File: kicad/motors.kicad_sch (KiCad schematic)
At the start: 61 parts, among them J12 Conn_01x04_Pin, J3 Conn_01x04_Pin, J4 Conn_01x04_Pin, J5 Conn_01x04_Pin, J6 Conn_01x04_Pin, U3 DRV8825PWP, U4 DRV8825PWP, U5 DRV8825PWP, U6 DRV8825PWP

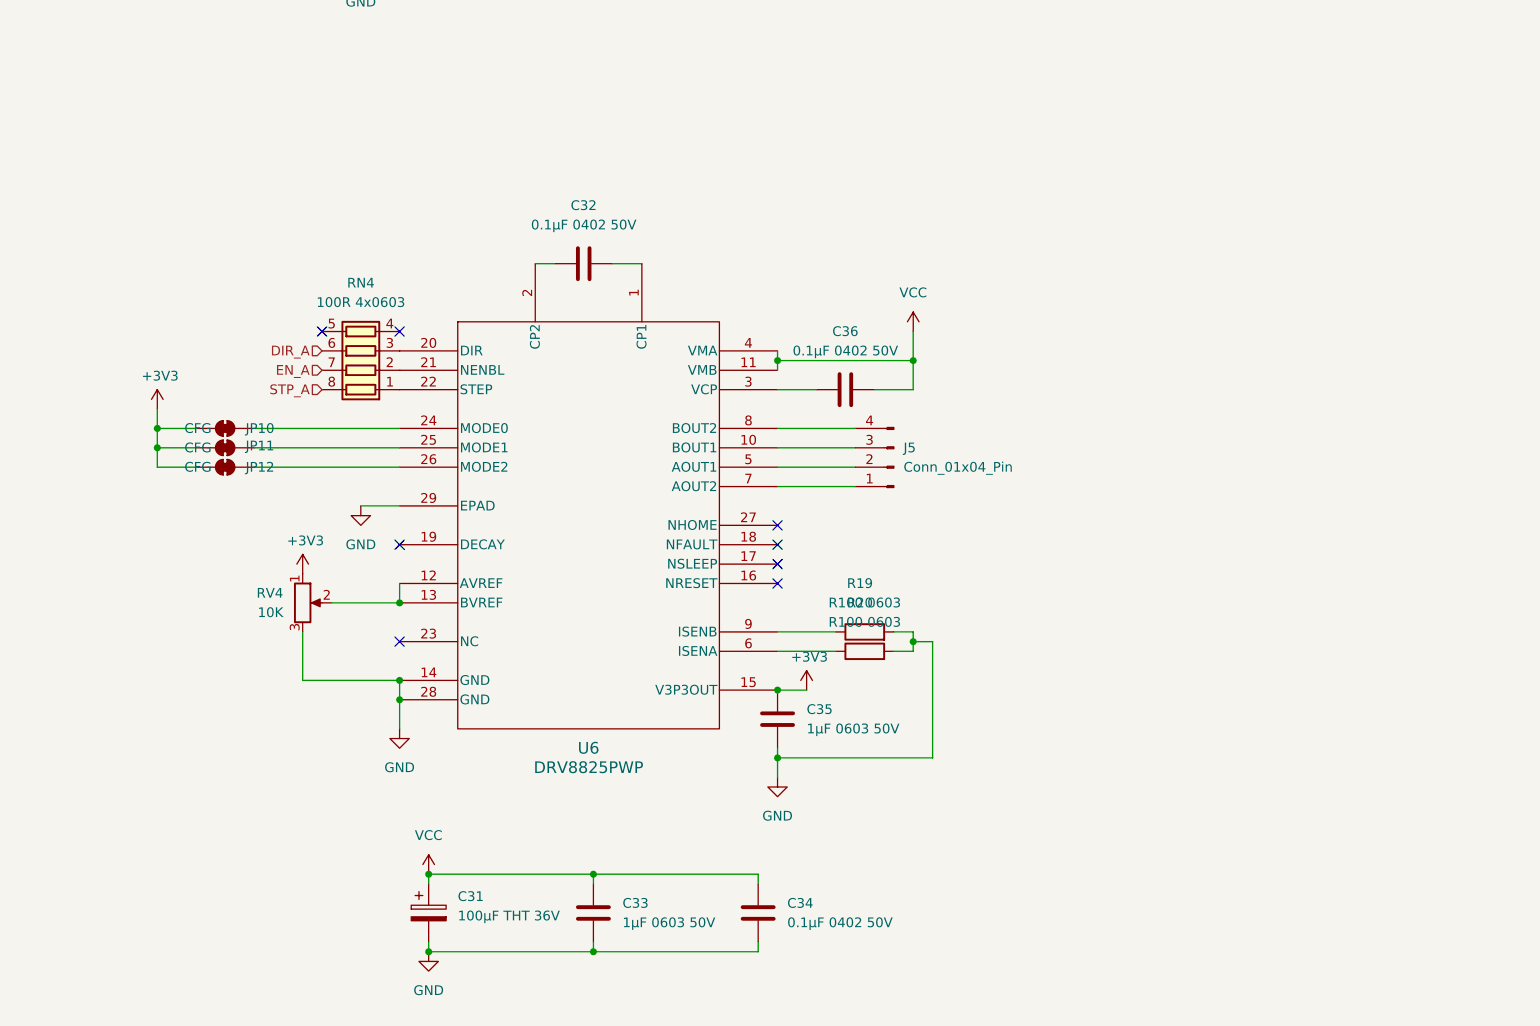
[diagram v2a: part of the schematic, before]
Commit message: Toshiba TB67S109A stepper driver
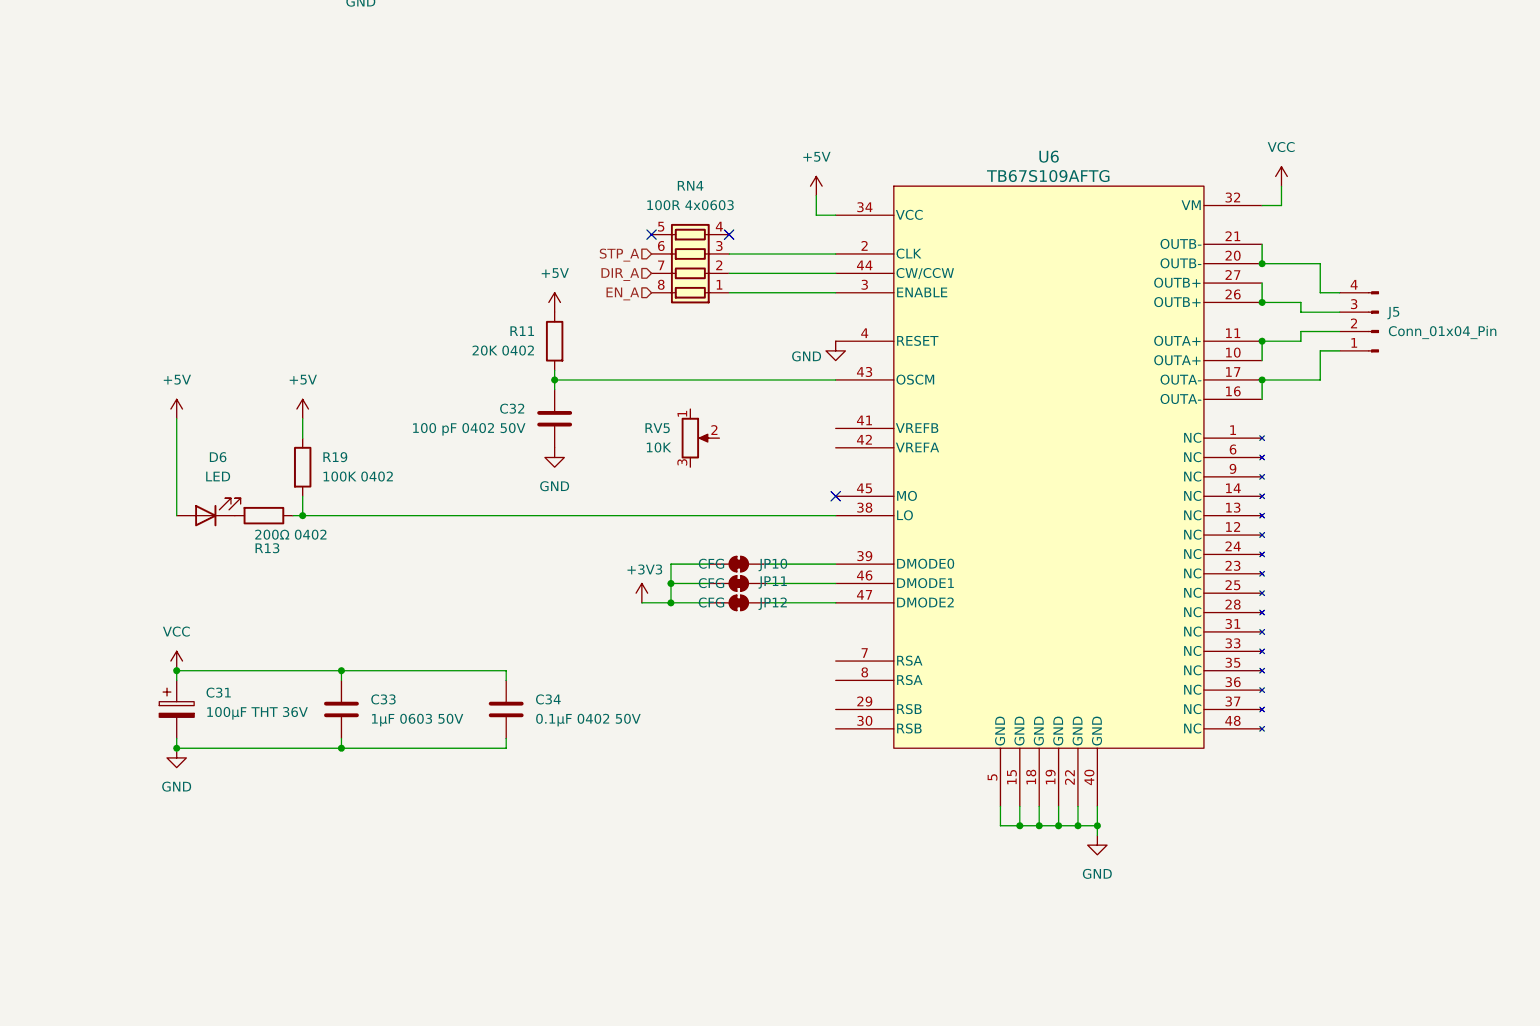
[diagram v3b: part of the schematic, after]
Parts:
- removed C35: 1μF 0603 50V, Capacitor_SMD:C_0402_1005Metric, symbol Device:C
- removed C36: 0.1μF 0402 50V, Capacitor_SMD:C_0402_1005Metric, symbol Device:C
- removed R20: R100 0603, Resistor_SMD:R_0603_1608Metric, symbol Device:R
- removed RV4: 10K, Potentiometer_SMD:Potentiometer_Bourns_TC33X_Vertical, symbol Device:R_Potentiometer
- removed U6: DRV8825PWP, Package_SO:HTSSOP-28-1EP_4.4x9.7mm_P0.65mm_EP3.4x9.5mm_ThermalVias, symbol rephat-symbols:DRV8825PWP
- added D6: LED, LED_SMD:LED_0603_1608Metric, symbol Device:LED
- added R11: 20K 0402, Resistor_SMD:R_0402_1005Metric, symbol Device:R
- added R13: 200Ω 0402, Resistor_SMD:R_0402_1005Metric, symbol Device:R
- added RV5: 10K, Potentiometer_SMD:Potentiometer_Bourns_TC33X_Vertical, symbol Device:R_Potentiometer
- added U6: TB67S109AFTG, Package_DFN_QFN:QFN-48-1EP_7x7mm_P0.5mm_EP5.45x5.45mm_ThermalVias, symbol rephat-symbols:TB67S109AFTG
- C32: value 0.1μF 0402 50V -> 100 pF 0402 50V
- R19: value R100 0603 -> 100K 0402; footprint Resistor_SMD:R_0603_1608Metric -> Resistor_SMD:R_0402_1005Metric
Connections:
- net DIR_A: now also RN4.7 (R2.2); no longer RN4.6 (R3.2)
- net EN_A: now also RN4.8 (R1.2); no longer RN4.7 (R2.2)
- net GND: now also C32.2, U6.15 (GND), U6.18 (GND), U6.19 (GND), U6.22 (GND), U6.4 (RESET), U6.40 (GND), U6.5 (GND); no longer R19.2
- net STP_A: now also RN4.6 (R3.2); no longer RN4.8 (R1.2)
- net VCC: now also U6.32 (VM)
- net at RN4.1 (R1.1): now also U6.3 (ENABLE)
- net at RN4.2 (R2.1): now also U6.44 (CW/CCW)
- net at RN4.3 (R3.1): now also U6.2 (CLK)
- net at JP10.2 (B): now also U6.39 (DMODE0)
- net +5V: now reaches R19.1
- net +5V: now also D6.2 (A), R11.1, U6.34 (VCC)
- net at J5.1 (Pin_1): now also U6.16 (OUTA-), U6.17 (OUTA-)
- net at J5.2 (Pin_2): now also U6.10 (OUTA+), U6.11 (OUTA+)
- net at J5.3 (Pin_3): now also U6.26 (OUTB+), U6.27 (OUTB+)
- net at J5.4 (Pin_4): now also U6.20 (OUTB-), U6.21 (OUTB-)
- net at JP11.2 (B): now also U6.46 (DMODE1)
- net at JP12.2 (B): now also U6.47 (DMODE2)
- net at C32.1: now also R11.2, U6.43 (OSCM)
- new net: R13.1, R19.2, U6.38 (LO)
- new net: D6.1 (K), R13.2
- no-connect marks 32 -> 27
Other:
- moved on the sheet: C31, C33, C34, J5, JP10, JP11, JP12, RN4
